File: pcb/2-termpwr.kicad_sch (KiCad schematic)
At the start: 0 parts

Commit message: Phase 3: populate TERMPWR sheet; schematic generator in pcb/_gen
TERMPWR sheet: CC detection (LM393 against a CJ431 2.5 V shunt
reference divided to 0.653 V, with hysteresis), the active-low
TERMPWR enable node (comparators wired-OR with the bench-present
FET), and the TERMPWR eFuse with its OVLO-as-enable divider, jumper,
TVS and indicator LEDs. Includes the owner's CJ431 and PWR_FLAG notes.

pcb/_gen regenerates the generated sheets and checks them against
KiCad's netlist. It refuses to overwrite a sheet edited in KiCad
since the last build (content fingerprints). Adds a CJ431 symbol
with JCET's pinout, and restores the USB_HS net-class patterns that
a KiCad save had dropped.
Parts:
- added C201, C202, C207: 1uF 25V, Capacitor_SMD:C_0402_1005Metric, symbol Device:C
- added C203, C206: 100nF 50V, Capacitor_SMD:C_0402_1005Metric, symbol Device:C
- added C204: 2.2nF, Capacitor_SMD:C_0402_1005Metric, symbol Device:C
- added C205: 1nF, Capacitor_SMD:C_0402_1005Metric, symbol Device:C
- added D201: KT-0603R red, LED_SMD:LED_0603_1608Metric, symbol Device:LED
- added D202: KT-0805Y yellow, LED_SMD:LED_0805_2012Metric, symbol Device:LED
- added D203: SS14, Diode_SMD:D_SMA, symbol Device:D_Schottky
- added D204: SMF6.0A, Diode_SMD:D_SMF, symbol Device:D_Zener
- added J201: TERMPWR jumper, Connector_PinHeader_2.54mm:PinHeader_1x02_P2.54mm_Vertical, symbol Connector_Generic:Conn_01x02
- added Q201: 2N7002, Package_TO_SOT_SMD:SOT-23, symbol Transistor_FET:2N7002
- added R201, R202, R204, R208, R210, R212: 10k, Resistor_SMD:R_0402_1005Metric, symbol Device:R
- added R203: 470R, Resistor_SMD:R_0402_1005Metric, symbol Device:R
- added R205: 3.3k, Resistor_SMD:R_0402_1005Metric, symbol Device:R
- added R206: 4.7k, Resistor_SMD:R_0402_1005Metric, symbol Device:R
- added R207: 1M, Resistor_SMD:R_0402_1005Metric, symbol Device:R
- added R209: 1k, Resistor_SMD:R_0402_1005Metric, symbol Device:R
- added R211: 100k, Resistor_SMD:R_0402_1005Metric, symbol Device:R
- added R213: 39k, Resistor_SMD:R_0402_1005Metric, symbol Device:R
- added R214: 15k, Resistor_SMD:R_0402_1005Metric, symbol Device:R
- added R215: 56k, Resistor_SMD:R_0402_1005Metric, symbol Device:R
- added R216: 47k, Resistor_SMD:R_0402_1005Metric, symbol Device:R
- added R217: 2.4k, Resistor_SMD:R_0402_1005Metric, symbol Device:R
- added R218: 330R, Resistor_SMD:R_0402_1005Metric, symbol Device:R
- added U201: TPS259470ARPWR, symbol scsi-adapter:TPS259470A
- added U202: LM393DR2G, Package_SO:SOIC-8_3.9x4.9mm_P1.27mm, symbol Comparator:LM393
- added U203: CJ431, Package_TO_SOT_SMD:SOT-23, symbol scsi-adapter:CJ431
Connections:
- net BENCH_5V: now also R210.1
- net CC1: now also R201.1
- net CC2: now also R202.1
- net TERMPWR_EFUSE_FAULT_INVERTED: now also U201.4 (~{FLT})
- net TERMPWR_EN_INVERTED: now also D201.1 (K), Q201.3 (D), R207.1, R208.2, R215.1, U202.1, U202.7
- new net: R204.2, R205.1
- new net: Q201.1 (G), R210.2, R211.1
- new net: D202.2 (A), R212.2
- new net: D201.2 (A), R209.2
- new net: C205.1, U201.10 (ITIMER)
- new net: C204.1, U201.7 (DVDT)
- new net: R217.2, R218.1
- new net: R217.1, U201.9 (ILM)
- new net +3V3: R203.1, R208.1, R209.1
- new net +5V_SYS: C203.1, C206.1, R213.1, U201.5 (IN), U202.8 (V+)
- new net CC1_FILTERED: C201.1, R201.2, U202.2 (-)
- new net CC2_FILTERED: C202.1, R202.2, U202.6 (-)
- new net CC_REFERENCE_2V5: R203.2, R204.1, U203.1 (REF), U203.2 (K)
- new net CC_THRESHOLD: R205.2, R206.1, R207.2, U202.3 (+), U202.5 (+)
- new net GND: C201.2, C202.2, C203.2, C204.2, C205.2, C206.2, C207.2, D202.1 (K), D203.2 (A), D204.2 (A), Q201.2 (S), R206.2, R211.2, R214.2, R216.2, R218.2, U201.8 (GND), U202.4 (V-), U203.3 (A)
- new net TERMPWR: D204.1 (K), J201.2 (Pin_2), R212.1
- new net TERMPWR_EFUSE_EN: R213.2, R214.1, U201.1 (EN/UVLO)
- new net TERMPWR_EFUSE_OUT: C207.1, D203.1 (K), J201.1 (Pin_1), U201.6 (OUT)
- new net TERMPWR_EFUSE_OV: R215.2, R216.1, U201.2 (OVLO)
- no-connect marks 0 -> 1
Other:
- note added: "0.653 V"
- note added: "1.11 V"
- note added: "2.50 V"
- note added: "CC voltage across our 5.1k Rd (usb-hub sheet): default USB <= 0.61 V, 1.5 A >= 0.70 V, 3 A >= 1.23 V. Only one CC is active (plug orientation), so each gets a comparator; the open-collector outputs are wired together. CC above CC_THRESHOLD -> output pulls TERMPWR_EN_INVERTED low. R207 adds hysteresis: 0.661 V rising / 0.651 V falling. Worst case (1 % R, +3V3 3.16-3.44 V, LM393 offset/bias, CJ431 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"
- note added: "CJ431 (U203) is a shunt regulator: it sinks current into its cathode (top) until its reference (side) sits at 2.500 V. REF is tied to the cathode, so the cathode is the 2.500 V output. It needs a bias resistor from the cathode to a supply, sized so it always gets at least 1 mA (its minimum for regulation). R203 470R from +3V3, nominal at 3.30 V: R203: (3.30 - 2.50) / 470 = 1.70 mA; R204-R206 (18.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"
- note added: "Current limit 1.22 A (1.06-1.39 A): >= 900 mA required, <= 1.5 A recommended (SCSI-2 5.4.3). True reverse blocking, even unpowered, so another device's TERMPWR can't back-feed the board."
- note added: "D203 DNP: TI suggests it against the negative spike when the eFuse cuts a long cable. Fit only if OUT dips below -0.8 V on the scope; its leakage counts against SCSI-2's 1 mA TERMPWR budget."
- note added: "Enabling through OVLO skips the dVdt ramp: TERMPWR rises at the 1.22 A limit (~0.2 ms into 50 uF). Harmless."
- note added: "Is the host port allowed to give us >= 1.5 A? If so, pull TERMPWR_EN_INVERTED low. Hardware only, no firmware."
- note added: "J201: shunt fitted = the board may supply TERMPWR (normal). Remove it to never drive TERMPWR, whatever CC or the bench say: e.g. another device already supplies it, or to isolate a TERMPWR fault (R2a)."
- note added: "Low = we supply TERMPWR. Wired-OR: either comparator (USB port offers >= 1.5 A) or Q201 (bench supply present)."
- note added: "OVLO as active-low enable: node high (~3.0 V) -> OVLO 1.31-1.43 V > 1.22 V: off. node low (<= 0.7 V) -> OVLO <= 0.32 V < 1.08 V: on."
- note added: "TERMPWR also arrives from other devices on the bus, hence the PWR_FLAG to tell KiCad that TERMPWR is powered from outside the drawn parts (through J201 and the bus), so ERC doesn't report 'power input not driven'. D202 (yellow) shows TERMPWR from anyone; D201 (red) shows that we supply it. Our non-terminator draw from TERMPWR: D202 0.35 mA + ADC divider (rp2350 sheet) 0.03 mA + eFuse leakage <= 0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"
- note added: "TERMPWR enable (TERMPWR_EN_INVERTED)"
- note added: "TERMPWR switch (eFuse)"
- note added: "USB-C current advertisement (CC detection)"
- note added: "UVLO: on above 1.20 x 54/15 = 4.32 V"
- note added: "With the TPS2116 in priority mode, 'bench present' also means the bench is powering the board. Q201's gate comes from the bench eFuse output (BENCH_5V), 4.5 V at 5 V, never the raw terminal. The node sits at ~3.0 V when high (R208 against the eFuse OVLO divider R215/R216), not 3.3 V. The expander reads this node (P01), so firmware can tell why TERMPWR is on or off. For a few ms at power-up (+5V_S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"
- note added: "eFuse setting pins: C204 on DVDT (dV/dt, output voltage slew rate): turn-on ramp, only at power-up; enabling through OVLO skips it. R217 + R218 on ILM (I-limit: sets the current limit, and the pin voltage doubles as a load-current monitor): 1.22 A (R = 3334 / I). 2.73k from two no-fee parts; a single 2.4k could reach 1.59 A. C205 on ITIMER (I-timer: overcurrent blanking timer), DNP. Open = limit 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"
- note removed: "TERMPWR (NOTES: TERMPWR, CC detection) TERMPWR eFuse TPS259470A (OVLO 56 k/47 k = active-low enable, ILIM 1.22 A, UVLO 4.32 V), CC detection LM393 + CJ431 reference + CC filters, bench-present 2N7002, enable-node pull-up, TERMPWR disable jumper, TERMPWR enable/present LEDs, SS14 (DNP), SMF6.0A ESD."

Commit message: Phase 3: footprint audit fixes and project footprint library
- New project footprint library pcb/scsi-adapter.pretty, generated by
  pcb/_gen/footprints.py from datasheet land patterns: TI RPW0010A (U101/U201),
  Kangnex WJ500V (J101), TE AMPLIMITE .050 HD50 (J302), SHOU HAN TF PUSH
  microSD (J501), Abracon AOTA-B201610 polarized inductor (L401), SHOU HAN
  2-pos DIP (SW301). fp-lib-table added.
- J303 LA header: 2x17 box header C20920, pins 33/34 NC (34-way ribbon to a
  future 2x16 adapter board).
- J302 HD50: TE 5787082-5 squeeze-latch receptacle; shielded symbol, shell to
  GND via R343 0R. TE STEP model git-ignored (pcb/scsi-adapter.3dshapes/).
- D101/D204/D605: D_SMF -> D_SOD-123F (parts are SOD-123FL).
- L401 pins swapped so pad 1 = polarity dot = DVDD_1V1 (RP2350 Fig. 23).
- SW401/SW402: Hroparts K2-1102DP C110153 on SW_PUSH_6mm.
- NOTES, decisions, sources updated; J601 pad question closed; RP2350B
  minimal-design layout copy planned (open question 17).
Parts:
- D204: footprint Diode_SMD:D_SMF -> Diode_SMD:D_SOD-123F
- U201: footprint (none) -> scsi-adapter:Texas_RPW0010A_VQFN-HR-10_2x2mm_P0.45mm
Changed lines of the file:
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@@
 		(property "Reference" "U201" (at 147.32 181.61 0) (effects (font (size 1.27 1.27)) (justify left)))
 		(property "Value" "TPS259470ARPWR" (at 177.8 181.61 0) (effects (font (size 1.27 1.27)) (justify right)))
-		(property "Footprint" "" (at 162.56 190.5 0) (effects (font (size 1.27 1.27)) (hide yes)))
+		(property "Footprint" "scsi-adapter:Texas_RPW0010A_VQFN-HR-10_2x2mm_P0.45mm" (at 162.56 190.5 0) (effects (font (size 1.27 1.27)) (hide yes)))
 		(property "Datasheet" "https://www.ti.com/lit/ds/symlink/tps25947.pdf" (at 162.56 190.5 0) (effects (font (size 1.27 1.27)) (hide yes)))
-		(property "Description" "TERMPWR eFuse. RPW QFN-10 footprint to do." (at 162.56 190.5 0) (effects (font (size 1.27 1.27)) (hide yes)))
+		(property "Description" "TERMPWR eFuse" (at 162.56 190.5 0) (effects (font (size 1.27 1.27)) (hide yes)))
 		(property "LCSC" "C3662799" (at 162.56 190.5 0) (effects (font (size 1.27 1.27)) (hide yes)))
 		(property "Fit" "JLC" (at 162.56 190.5 0) (effects (font (size 1.27 1.27)) (hide yes)))
@@
 		(property "Reference" "D204" (at 347.98 195.58 270) (effects (font (size 1.27 1.27)) (justify right)))
 		(property "Value" "SMF6.0A" (at 347.98 198.12 270) (effects (font (size 1.27 1.27)) (justify right)))
-		(property "Footprint" "Diode_SMD:D_SMF" (at 345.44 196.85 0) (effects (font (size 1.27 1.27)) (hide yes)))
+		(property "Footprint" "Diode_SMD:D_SOD-123F" (at 345.44 196.85 0) (effects (font (size 1.27 1.27)) (hide yes)))
 		(property "Datasheet" "" (at 345.44 196.85 0) (effects (font (size 1.27 1.27)) (hide yes)))
 		(property "Description" "TERMPWR ESD / TVS" (at 345.44 196.85 0) (effects (font (size 1.27 1.27)) (hide yes)))

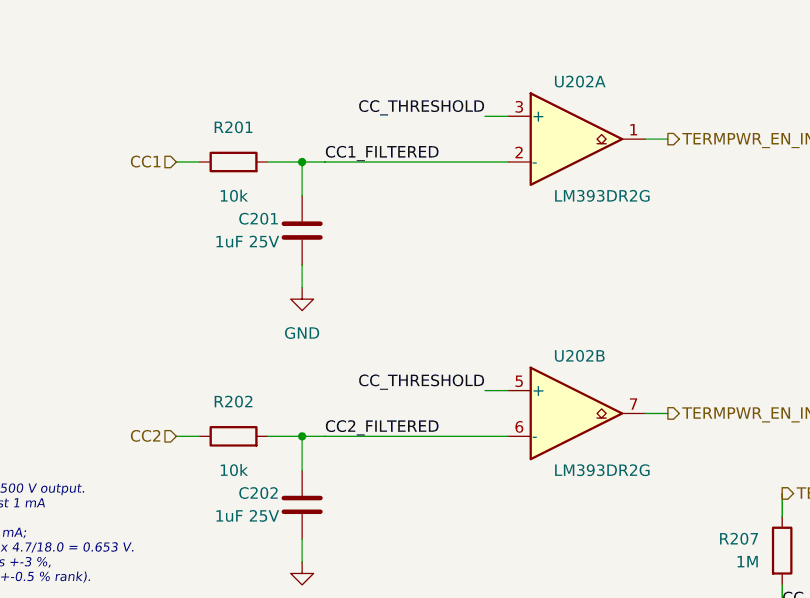
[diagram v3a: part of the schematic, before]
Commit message: route more scsi traces
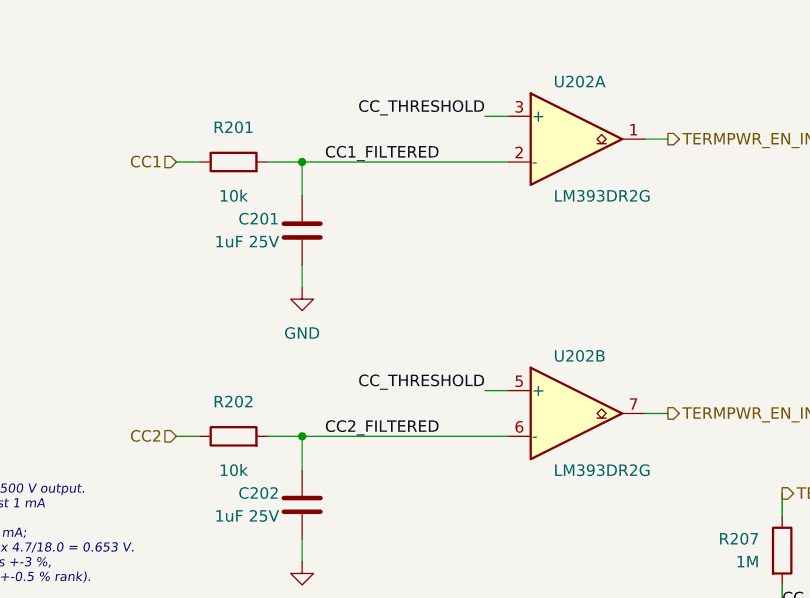
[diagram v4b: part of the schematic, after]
